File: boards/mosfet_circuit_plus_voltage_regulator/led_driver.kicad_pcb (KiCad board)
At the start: 2 copper layers, 25 parts, among them J1 Vin, J2 LED, J3 control_in, Q1 N_chan_mosfet, Q2 P-Chan_mosfet, U1 MC34063AP

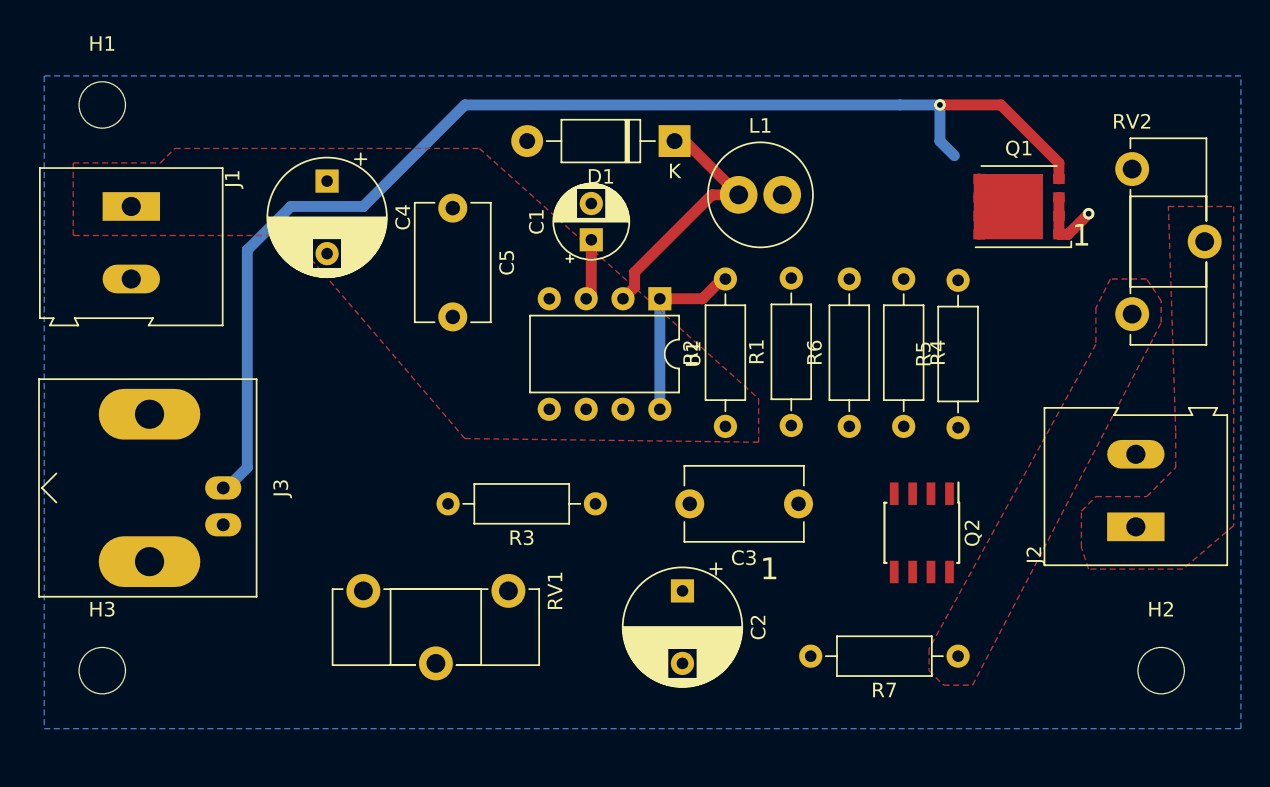
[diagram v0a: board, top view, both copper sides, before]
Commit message: final first draft of new board. now to order it and test
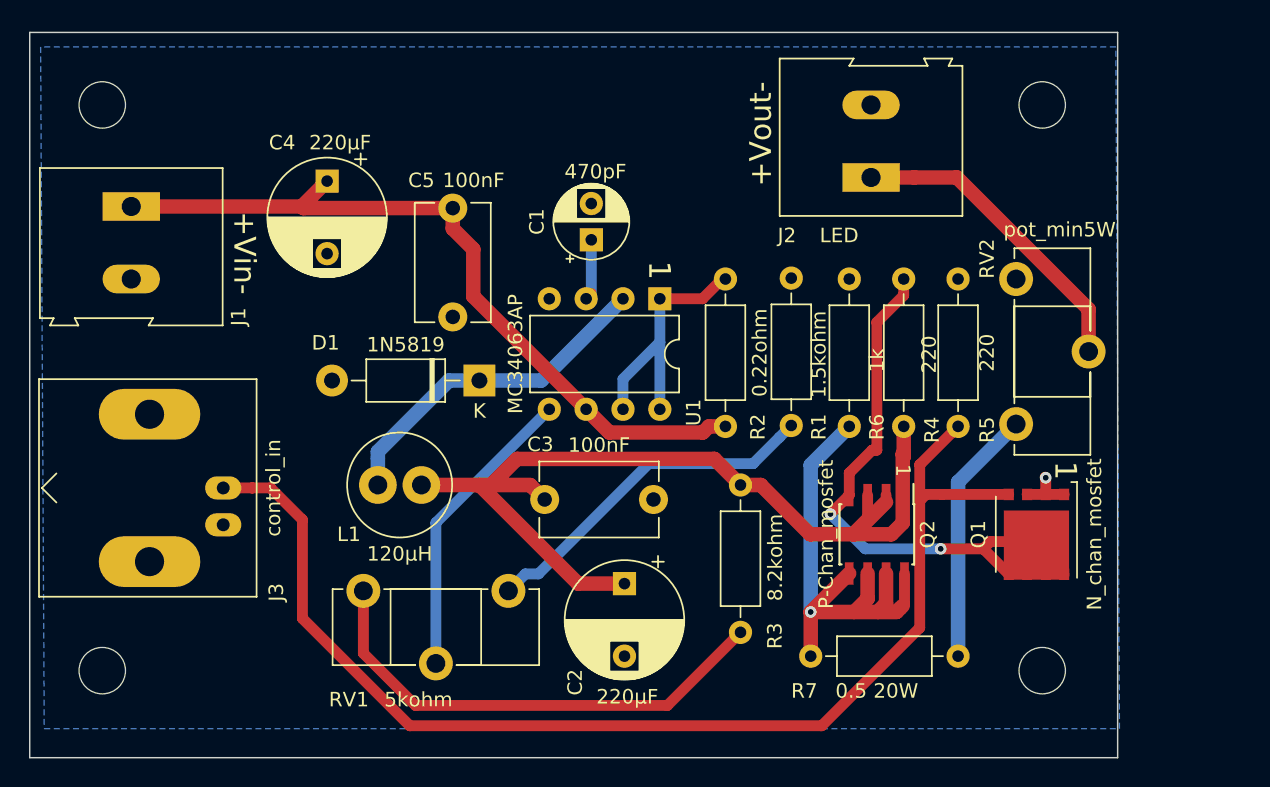
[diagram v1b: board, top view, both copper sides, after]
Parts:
- added H4: MountingHole, MountingHole:MountingHole_3.2mm_M3, F.Cu at (155.8, 58.0)
- moved L1 31.9 mm to (110.0, 84.2)
- moved J2 30.2 mm to (144.0, 63.0)
- moved Q1 22.6 mm to (155.4, 87.6), turned to 270 degrees
- moved D1 21.3 mm to (117.0, 77.0)
- moved RV2 11.0 mm to (154.0, 70.0)
- moved R5 10.2 mm to (150.0, 70.0), turned to 270 degrees
- moved R3 10.1 mm to (135.0, 84.2), turned to 270 degrees
- moved C3 10.0 mm to (129.0, 85.2)
- moved H2 8.20 mm to (155.8, 97.0)
- moved C2 4.03 mm to (127.0, 91.0)
- moved Q2 3.10 mm to (144.4, 87.6)
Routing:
- net Net-(C2-Pad1): track 0.00 -> 85.7 mm
- net VDD: track 0.00 -> 52.8 mm
- net Net-(Q2-Pad5): track 0.00 -> 35.4 mm, vias 0 -> 1
- net Net-(Q1-Pad5): track 6.34 -> 40.9 mm, vias 0 -> 2
- net Net-(R3-Pad2): track 0.00 -> 34.0 mm
- net Net-(R1-Pad1): track 0.00 -> 24.2 mm
- net Net-(J2-Pad1): track 0.00 -> 21.7 mm
- net Net-(RV1-Pad2): track 0.00 -> 20.8 mm
- net Net-(R7-Pad1): track 0.00 -> 17.7 mm
- net Net-(D1-Pad1): track 17.5 -> 23.6 mm
- net Net-(R2-Pad2): track 12.8 -> 18.5 mm
- net GND: track 5.19 -> 3.76 mm
- net Net-(J3-Pad1): track 84.0 -> 83.1 mm, vias 1 -> 0
- removed copper zone on F.Cu, net Net-(J2-Pad1)
- removed copper zone on F.Cu, net Net-(R7-Pad1)
- removed copper zone on F.Cu, net VDD
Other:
- board outline added: 75 x 50 mm
- net class power_line added: clearance 0.3, trace_width 1, via_dia 0.8, via_drill 0.4
- board text added: "+Vin-"
- board text added: "+Vout-"
